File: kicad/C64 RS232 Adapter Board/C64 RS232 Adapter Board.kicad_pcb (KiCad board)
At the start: 2 copper layers, 59.6 x 53.1 mm, 29 parts, among them J1 RS232_HDR, J2 DB25_RS232, J3 C64_USER_PORT, J4 User Port Breakout, SW1 RESET, U1 MAX3241ECAI+T

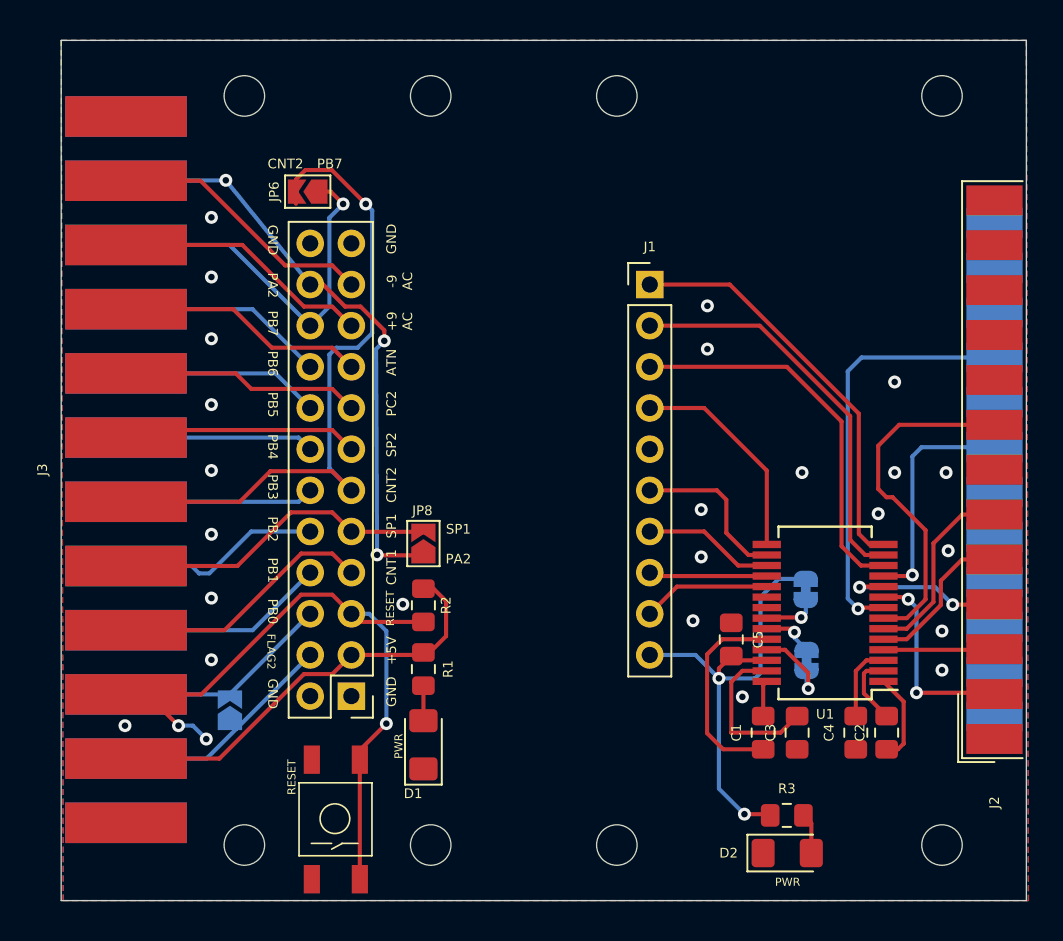
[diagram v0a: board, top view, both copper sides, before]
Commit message: rounded the corner yo
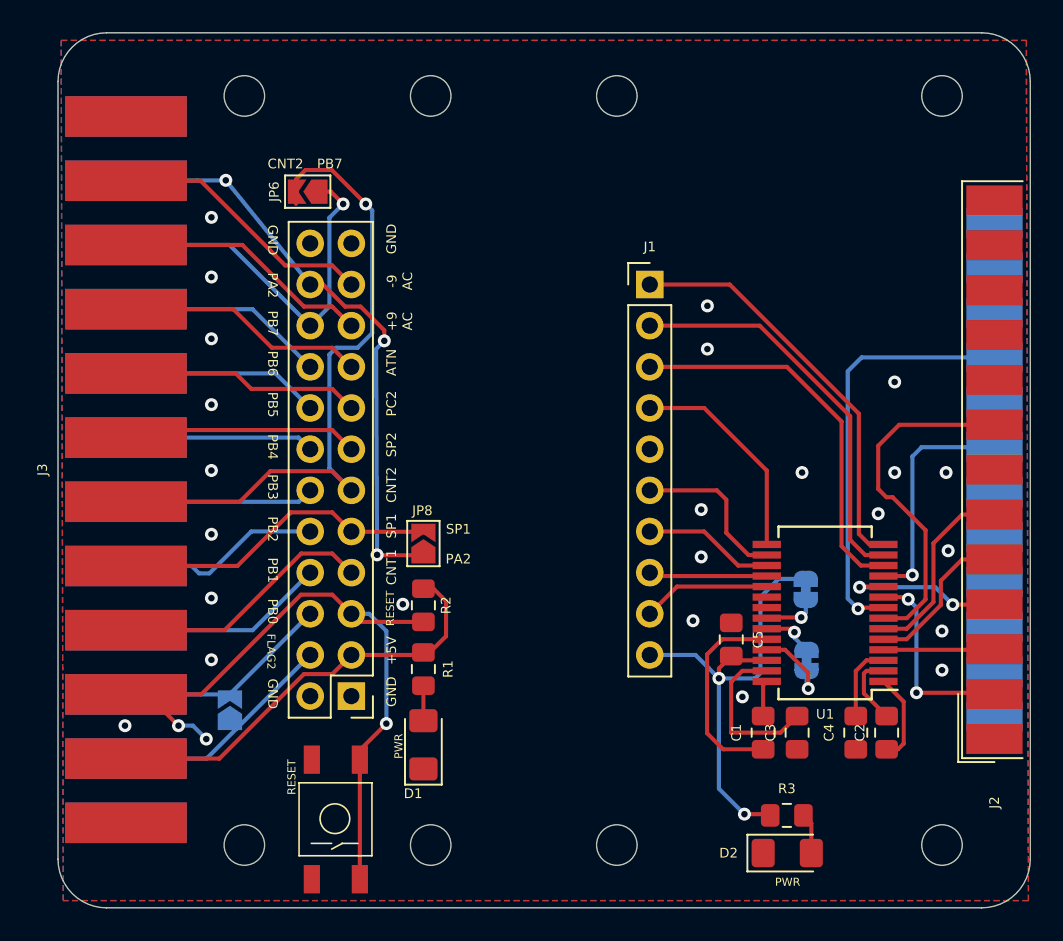
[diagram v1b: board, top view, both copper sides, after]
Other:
- board size 59.6 x 53.1 mm -> 60 x 54 mm
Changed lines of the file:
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@@
   (general
     (thickness 1.6)
-    (drawings 37)
+    (drawings 41)
     (tracks 306)
     (zones 0)
@@
     (46 B.CrtYd user)
     (47 F.CrtYd user)
-    (48 B.Fab user hide)
-    (49 F.Fab user hide)
+    (48 B.Fab user)
+    (49 F.Fab user)
   )
   (setup
@@
     (pad_to_mask_clearance 0.05)
     (aux_axis_origin 0 0)
-    (visible_elements 7FFFEFFF)
+    (visible_elements 7FFFF7FF)
     (pcbplotparams
       (layerselection 0x010fc_ffffffff)
@@
     (pad 1 np_thru_hole circle (at 0 0) (size 2.5 2.5) (drill 2.5) (layers *.Cu *.Mask))
   )
-  (gr_line (start 44.196 53.467) (end 103.759 53.467) (layer Edge.Cuts) (width 0.05))
-  (gr_line (start 44.196 106.553) (end 44.196 53.467) (layer Edge.Cuts) (width 0.05))
-  (gr_line (start 103.759 106.553) (end 44.196 106.553) (layer Edge.Cuts) (width 0.05))
-  (gr_line (start 103.759 53.467) (end 103.759 106.553) (layer Edge.Cuts) (width 0.05))
+  (gr_line (start 47 53) (end 101 53) (layer Edge.Cuts) (width 0.05))
+  (gr_line (start 44 104) (end 44 56) (layer Edge.Cuts) (width 0.05))
+  (gr_line (start 101 107) (end 47 107) (layer Edge.Cuts) (width 0.05))
+  (gr_line (start 104 56) (end 104 104) (layer Edge.Cuts) (width 0.05))
+  (gr_arc (start 47 56) (end 47 53) (angle -90) (layer Edge.Cuts) (width 0.05))
+  (gr_arc (start 47 104) (end 44 104) (angle -90) (layer Edge.Cuts) (width 0.05))
+  (gr_arc (start 101 56) (end 104 56) (angle -90) (layer Edge.Cuts) (width 0.05))
+  (gr_arc (start 101 104) (end 101 107) (angle -90) (layer Edge.Cuts) (width 0.05))
   (gr_text PWR (at 89.027 105.41) (layer F.SilkS)
     (effects (font (size 0.5 0.5) (thickness 0.1)))
